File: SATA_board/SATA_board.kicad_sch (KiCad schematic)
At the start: 7 parts, among them J1 47018-2001, J2 47018-2001, J3 678008025, J4 678008025, J6 47053-1000, J7 47053-1000, U1 LM5175RHF

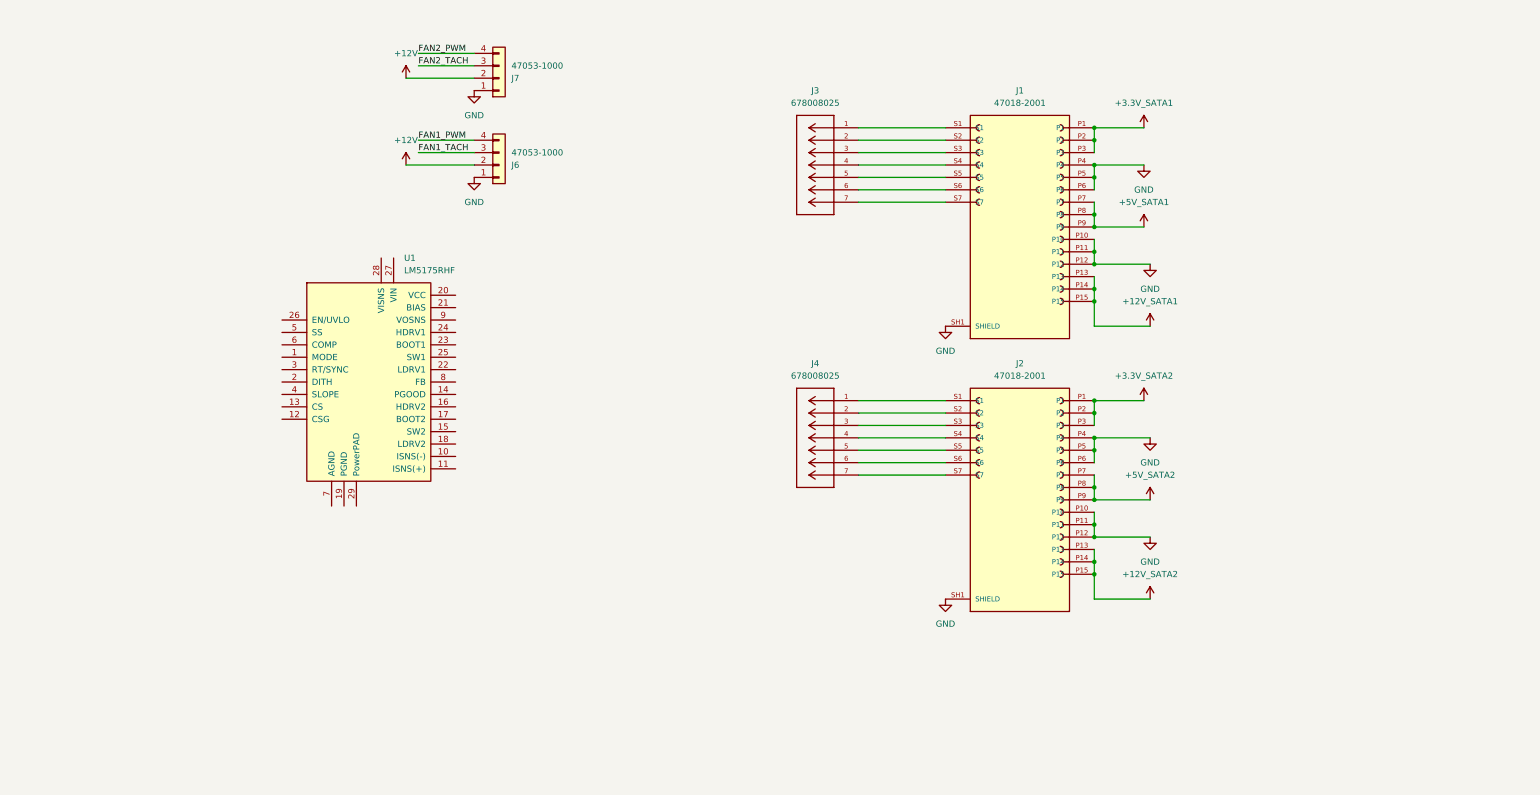
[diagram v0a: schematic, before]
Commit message: work
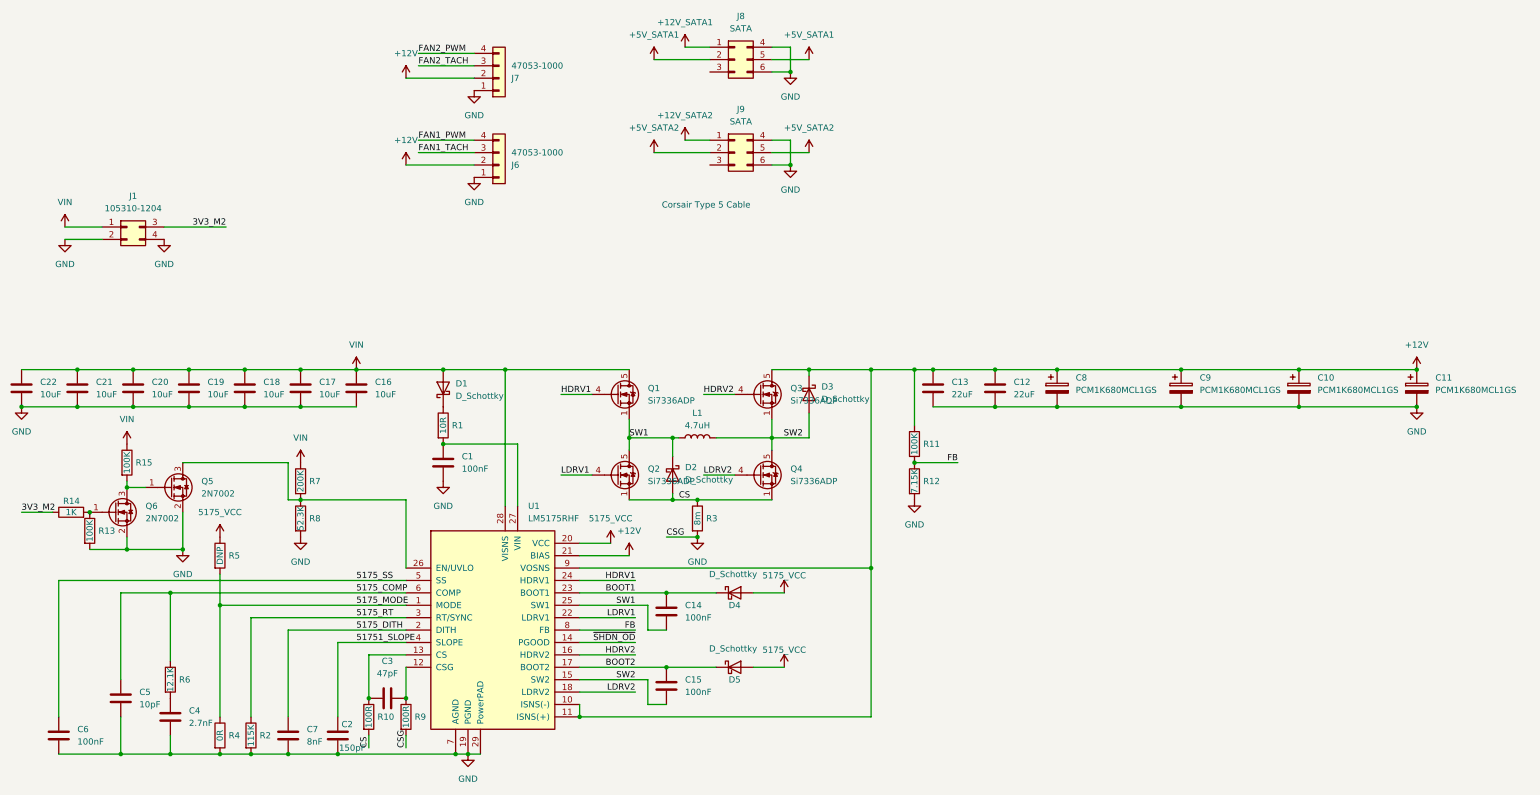
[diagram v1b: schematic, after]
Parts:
- removed J1, J2: 47018-2001, 47018-2001:MOLEX_47018-2001, symbol 47018-2001:47018-2001
- removed J3, J4: 678008025, 678008025:CONN_67800-8025_MOL, symbol 678008025:678008025
- added C1, C14, C15, C6: 100nF, symbol Device:C
- added C10, C11, C8, C9: PCM1K680MCL1GS, Capacitor_SMD:CP_Elec_10x10, symbol Device:C_Polarized
- added C12, C13: 22uF, symbol Device:C
- added C16, C17, C18, C19, C20, C21, C22: 10uF, symbol Device:C
- added C2: 150pF, symbol Device:C
- added C3: 47pF, symbol Device:C
- added C4: 2.7nF, symbol Device:C
- added C5: 10pF, symbol Device:C
- added C7: 8nF, symbol Device:C
- added D1, D2, D3, D4, D5: D_Schottky, symbol Device:D_Schottky
- added J1: 105310-1204, Connector_Molex:Molex_Nano-Fit_105310-xx04_2x02_P2.50mm_Vertical, symbol Connector_Generic:Conn_02x02_Top_Bottom
- added J8, J9: SATA, Connector_Molex:Molex_Micro-Fit_3.0_43045-0612_2x03_P3.00mm_Vertical, symbol Connector_Generic:Conn_02x03_Top_Bottom
- added L1: 4.7uH, symbol Device:L
- added Q1, Q2, Q3, Q4: Si7336ADP, Package_SO:PowerPAK_SO-8_Single, symbol Transistor_FET:Si7336ADP
- added Q5, Q6: 2N7002, Package_TO_SOT_SMD:SOT-23, symbol Transistor_FET:2N7002
- added R1: 10R, symbol Device:R
- added R10, R9: 100R, symbol Device:R
- added R11, R13, R15: 100K, symbol Device:R
- added R12: 7.15K, symbol Device:R
- added R14: 1K, symbol Device:R
- added R2: 115K, symbol Device:R
- added R3: 8m, symbol Device:R
- added R4: 0R, symbol Device:R
- added R5: DNP, symbol Device:R
- added R6: 12.1K, symbol Device:R
- added R7: 200K, symbol Device:R
- added R8: 52.3K, symbol Device:R
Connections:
- net +12V: now also U1.10 (ISNS(-)), U1.11 (ISNS(+)), U1.21 (BIAS), U1.9 (VOSNS), C10.1, C11.1, C12.1, C13.1, C8.1, C9.1, D3.1 (K), Q3.5 (D), R11.1
- net +12V_SATA1: now also J8.1 (Pin_1)
- net +12V_SATA2: now also J9.1 (Pin_1)
- net +5V_SATA1: now also J8.2 (Pin_2), J8.5 (Pin_5)
- net +5V_SATA2: now also J9.2 (Pin_2), J9.5 (Pin_5)
- net GND: now also U1.19 (PGND), U1.29 (PowerPAD), U1.7 (AGND), C1.2, C10.2, C11.2, C12.2, C13.2, C16.2, C17.2, C18.2, C19.2, C2.2, C20.2, C21.2, C22.2, C4.2, C5.2, C6.2, C7.2, C8.2, C9.2, J1.2 (Pin_2), J1.4 (Pin_4), J8.4 (Pin_4), J8.6 (Pin_6), J9.4 (Pin_4), J9.6 (Pin_6), Q5.2 (S), Q6.2 (S), R12.2, R13.2, R2.2, R3.2, R4.2, R8.2, R9.2
- net 5175_MODE: now reaches U1.1 (MODE)
- net 5175_MODE: now also R4.1, R5.2
- net at U1.12 (CSG): now also C3.2, R9.1
- net at U1.13 (CS): now also C3.1, R10.1
- net ~{SHDN_OD}: now reaches U1.14 (PGOOD)
- net SW2: now reaches U1.15 (SW2)
- net SW2: now also C15.2, D3.2 (A), L1.2, Q3.1 (S), Q3.2 (S), Q3.3 (S), Q4.5 (D)
- net HDRV2: now reaches U1.16 (HDRV2)
- net HDRV2: now also Q3.4 (G)
- net BOOT2: now reaches U1.17 (BOOT2)
- net BOOT2: now also C15.1, D5.1 (K)
- net LDRV2: now reaches U1.18 (LDRV2)
- net LDRV2: now also Q4.4 (G)
- net 5175_DITH: now reaches U1.2 (DITH)
- net 5175_DITH: now also C7.1
- net 5175_VCC: now reaches U1.20 (VCC)
- net 5175_VCC: now also D4.2 (A), D5.2 (A), R5.1
- net LDRV1: now reaches U1.22 (LDRV1)
- net LDRV1: now also Q2.4 (G)
- net BOOT1: now reaches U1.23 (BOOT1)
- net BOOT1: now also C14.1, D4.1 (K)
- net HDRV1: now reaches U1.24 (HDRV1)
- net HDRV1: now also Q1.4 (G)
- net SW1: now reaches U1.25 (SW1)
- net SW1: now also C14.2, D2.1 (K), L1.1, Q1.1 (S), Q1.2 (S), Q1.3 (S), Q2.5 (D)
- net at U1.26 (EN/UVLO): now also Q5.3 (D), R7.2, R8.1
- net at U1.27 (VIN): now also C1.1, R1.2
- net VIN: now reaches U1.28 (VISNS)
- net VIN: now also C16.1, C17.1, C18.1, C19.1, C20.1, C21.1, C22.1, D1.2 (A), J1.1 (Pin_1), Q1.5 (D), R15.1, R7.1
- net 5175_RT: now reaches U1.3 (RT/SYNC)
- net 5175_RT: now also R2.1
- net 51751_SLOPE: now reaches U1.4 (SLOPE)
- net 51751_SLOPE: now also C2.1
- net 5175_SS: now reaches U1.5 (SS)
- net 5175_SS: now also C6.1
- net 5175_COMP: now reaches U1.6 (COMP)
- net 5175_COMP: now also C5.1, R6.1
- net FB: now reaches U1.8 (FB)
- net FB: now also R11.2, R12.1
- new net: Q6.1 (G), R13.1, R14.2
- new net: C4.1, R6.2
- new net: Q5.1 (G), Q6.3 (D), R15.2
- new net: D1.1 (K), R1.1
- new net 3V3_M2: J1.3 (Pin_3), R14.1
- new net CS: D2.2 (A), Q2.1 (S), Q2.2 (S), Q2.3 (S), Q4.1 (S), Q4.2 (S), Q4.3 (S), R10.2, R3.1
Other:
- note added: "Corsair Type 5 Cable"
- moved on the sheet: U1
